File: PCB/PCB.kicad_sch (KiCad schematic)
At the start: 0 parts

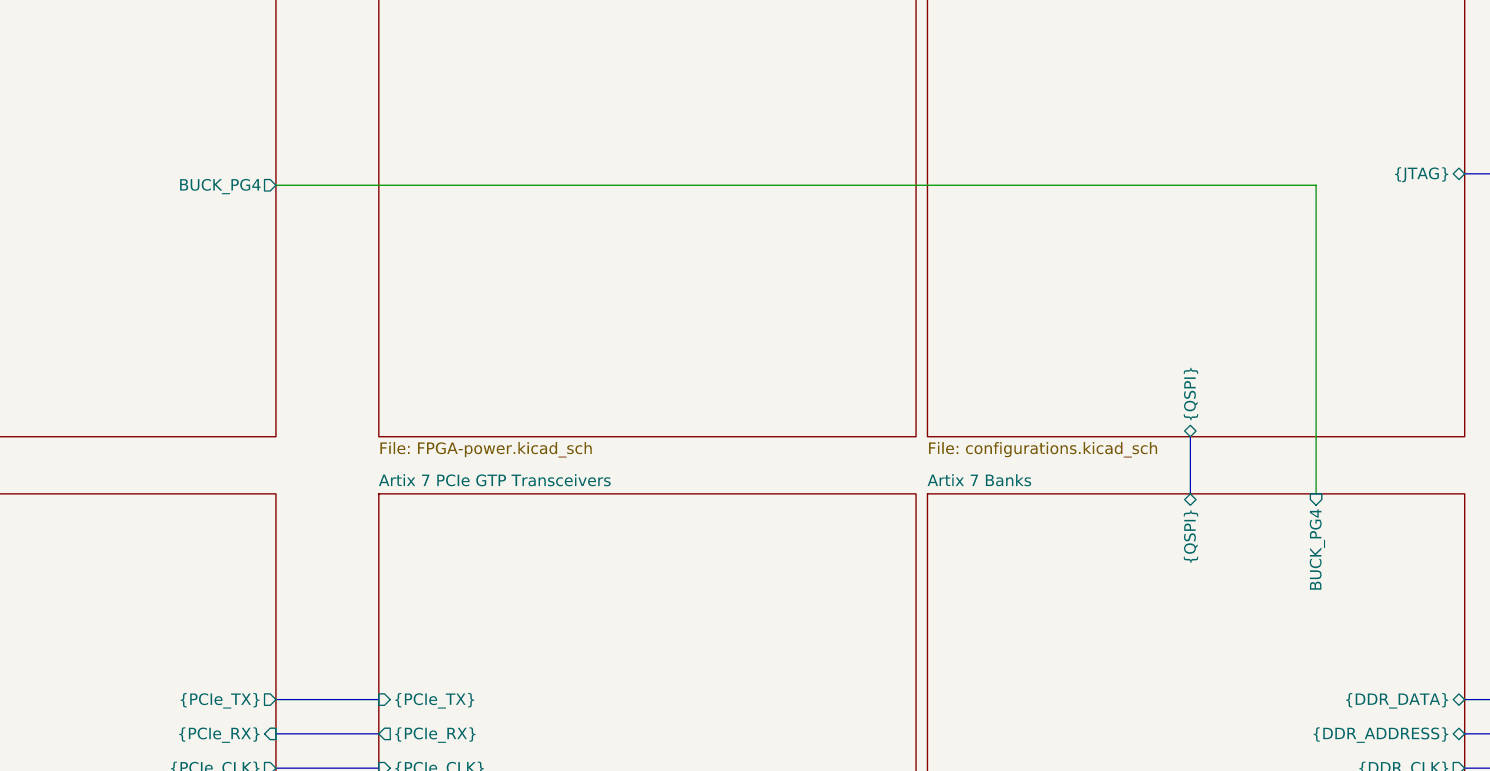
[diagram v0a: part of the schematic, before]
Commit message: completely finished the clock, cleaned up the schematic
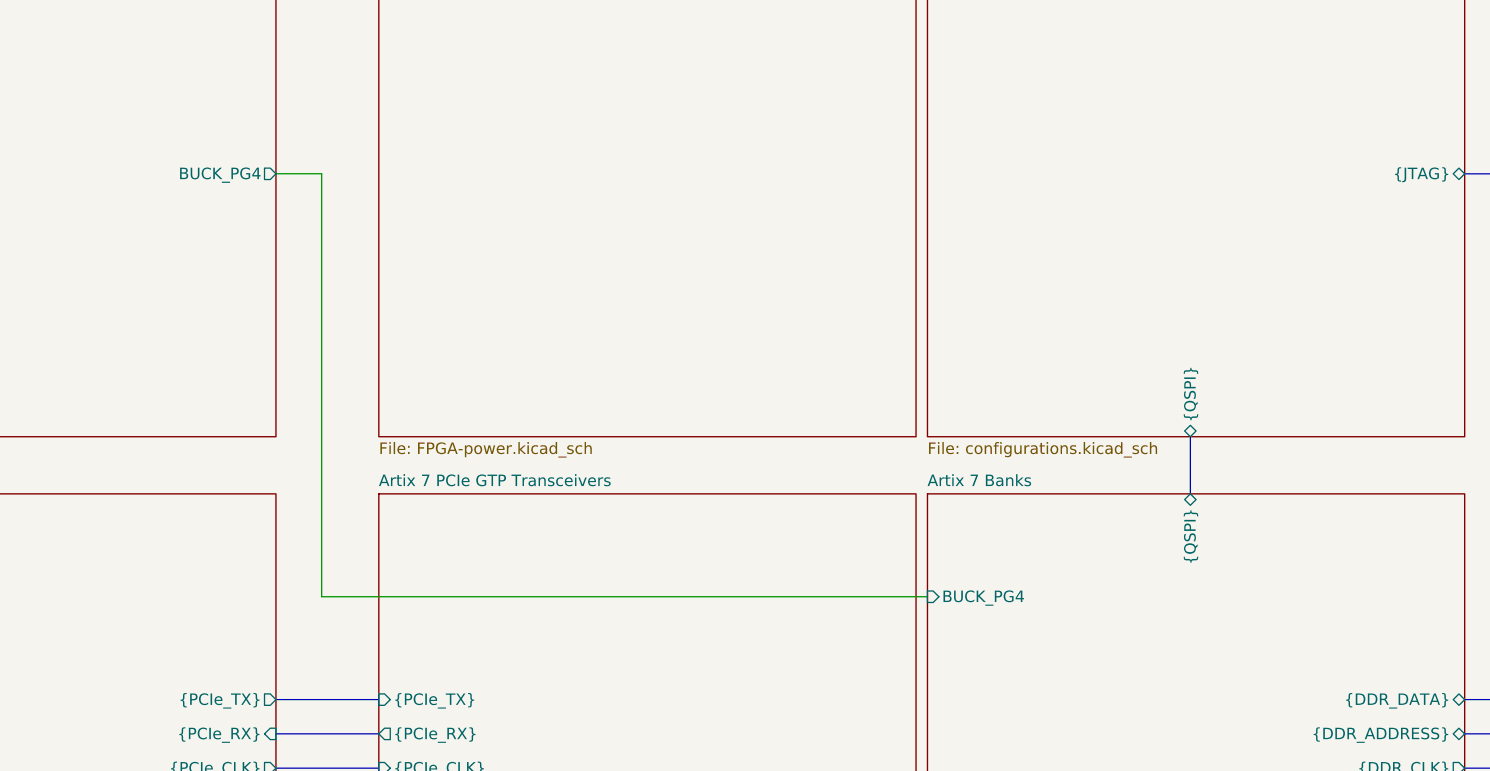
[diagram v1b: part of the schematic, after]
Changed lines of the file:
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@@
 	(wire
 		(pts
-			(xy 129.54 82.55) (xy 245.11 82.55)
+			(xy 134.62 81.28) (xy 134.62 128.27)
 		)
 		(stroke
@@
 	(wire
 		(pts
-			(xy 245.11 82.55) (xy 245.11 116.84)
+			(xy 134.62 128.27) (xy 201.93 128.27)
 		)
 		(stroke
@@
 		(pts
 			(xy 261.62 147.32) (xy 274.32 147.32)
+		)
+		(stroke
+			(width 0)
+			(type default)
+		)
+	)
+	(wire
+		(pts
+			(xy 129.54 81.28) (xy 134.62 81.28)
 		)
 		(stroke
@@
 		)
 		(pin "BUCK_PG4" output
-			(at 129.54 82.55 0)
+			(at 129.54 81.28 0)
 			(effects
 				(font
@@
 		)
 		(pin "BUCK_PG4" input
-			(at 245.11 116.84 90)
-			(effects
-				(font
-					(size 1.27 1.27)
-				)
-				(justify right)
-			)
-		)
+			(at 201.93 128.27 180)
+			(effects
+				(font
+					(size 1.27 1.27)
+				)
+				(justify left)
+			)
+		)
